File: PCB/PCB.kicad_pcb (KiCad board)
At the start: 2 copper layers, 8 parts, among them J1 Barrel_Jack_MountingPin, M1 Motor_Servo, M2 Motor_Servo, M3 Motor_Servo, M4 Motor_Servo, M5 Motor_Servo, M6 Motor_Servo, U1 ESP32-Devkit-V1

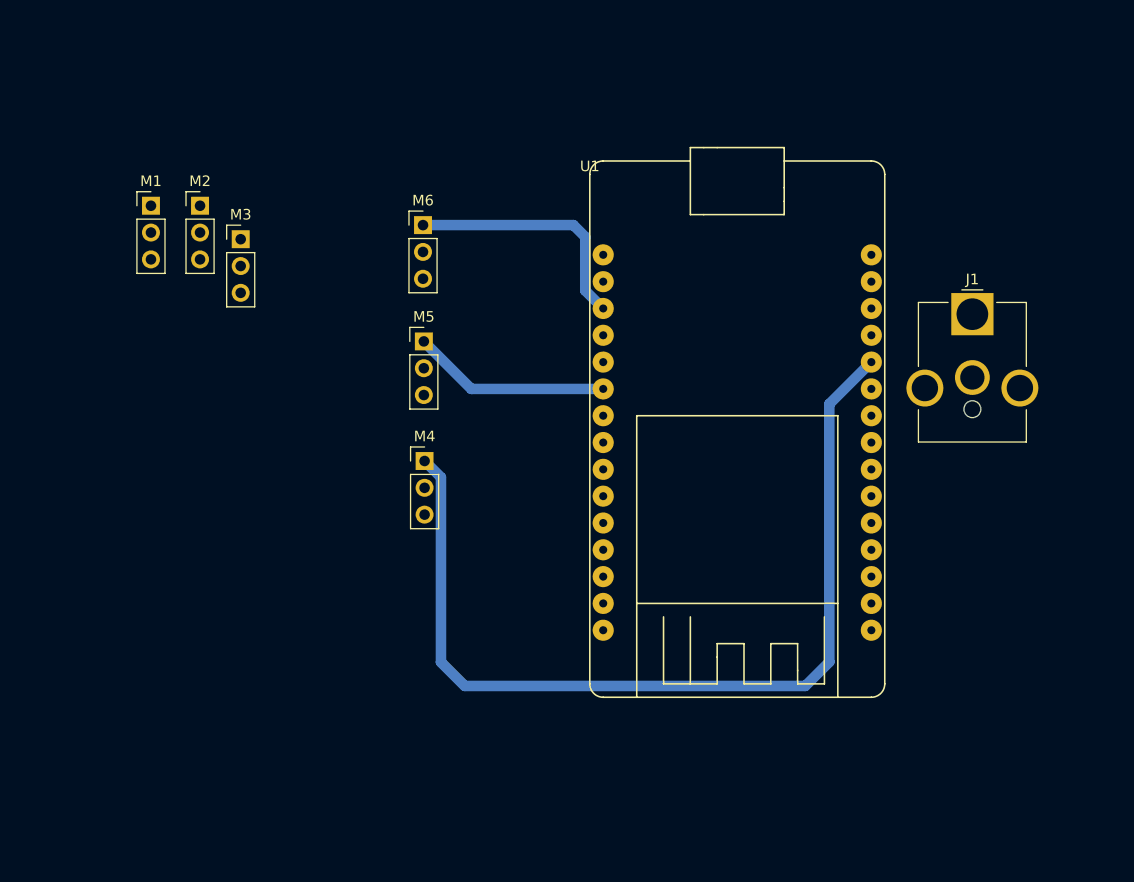
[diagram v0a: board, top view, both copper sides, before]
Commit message: Pcb para imprimir
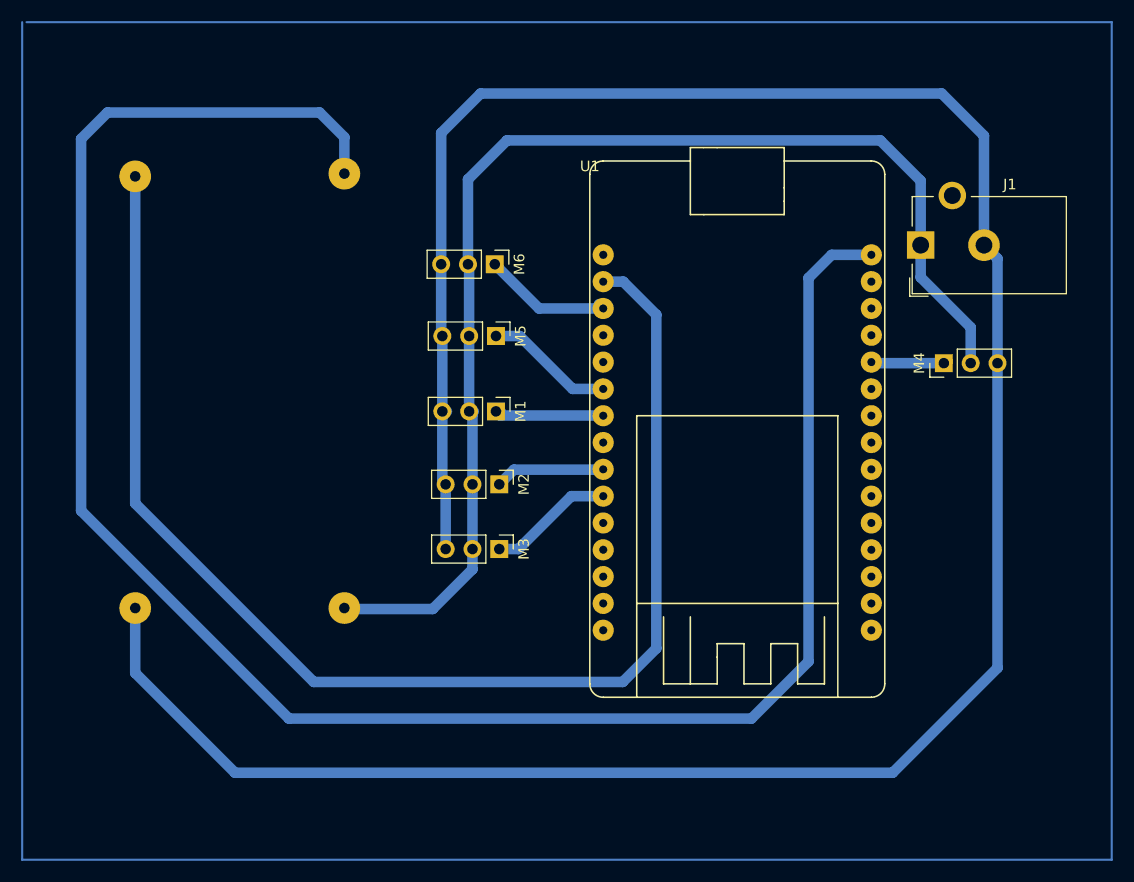
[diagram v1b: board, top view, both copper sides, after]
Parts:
- added U2: ~, Stepdown:Step down lm, F.Cu at (-15.1, -15.1)
- J1: footprint Connector_BarrelJack:BarrelJack_CUI_PJ-063AH_Horizontal_CircularHoles -> Connector_BarrelJack:BarrelJack_CUI_PJ-102AH_Horizontal
- moved M4 50.1 mm to (129.1, 115.8), turned to 90 degrees
- moved M2 38.7 mm to (87.0, 127.3), turned to -90 degrees
- moved M3 38.2 mm to (87.0, 133.4), turned to -90 degrees
- moved M1 38.0 mm to (86.6, 120.4), turned to -90 degrees
- moved J1 8.17 mm to (126.9, 104.7), turned to 90 degrees
- moved M6 7.74 mm to (86.5, 106.5), turned to -90 degrees
- moved M5 6.85 mm to (86.6, 113.3), turned to -90 degrees
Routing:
- net GND: track 0.00 -> 241.1 mm
- net VccPlaca: track 0.00 -> 188.1 mm
- net GndPlaca: track 0.00 -> 126.6 mm
- net +12V: track 0.00 -> 116.1 mm
- net PWM6: track 88.4 -> 7.02 mm
- net PWM1: track 0.00 -> 11.9 mm
- net PWM5: track 23.3 -> 12.6 mm
- net PWM2: track 0.00 -> 10.4 mm
- net PWM3: track 0.00 -> 10.3 mm
- net PWM4: track 18.9 -> 12.3 mm
